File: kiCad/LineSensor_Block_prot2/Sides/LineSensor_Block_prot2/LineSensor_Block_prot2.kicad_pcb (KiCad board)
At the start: 2 copper layers, 91.3 x 94.2 mm, 58 parts, among them J1 Conn_01x09_Socket, J10 Conn_01x03_Socket, J11 Conn_01x03_Socket, J12 Conn_01x03_Socket, J2 Conn_01x09_Socket, J9 Conn_01x03_Socket, Q1 Q_Photo_NPN, Q10 Q_Photo_NPN, Q11 Q_Photo_NPN, Q12 Q_Photo_NPN, Q2 Q_Photo_NPN, Q3 Q_Photo_NPN, Q4 Q_Photo_NPN, Q5 Q_Photo_NPN, Q6 Q_Photo_NPN, Q7 Q_Photo_NPN, Q8 Q_Photo_NPN, Q9 Q_Photo_NPN

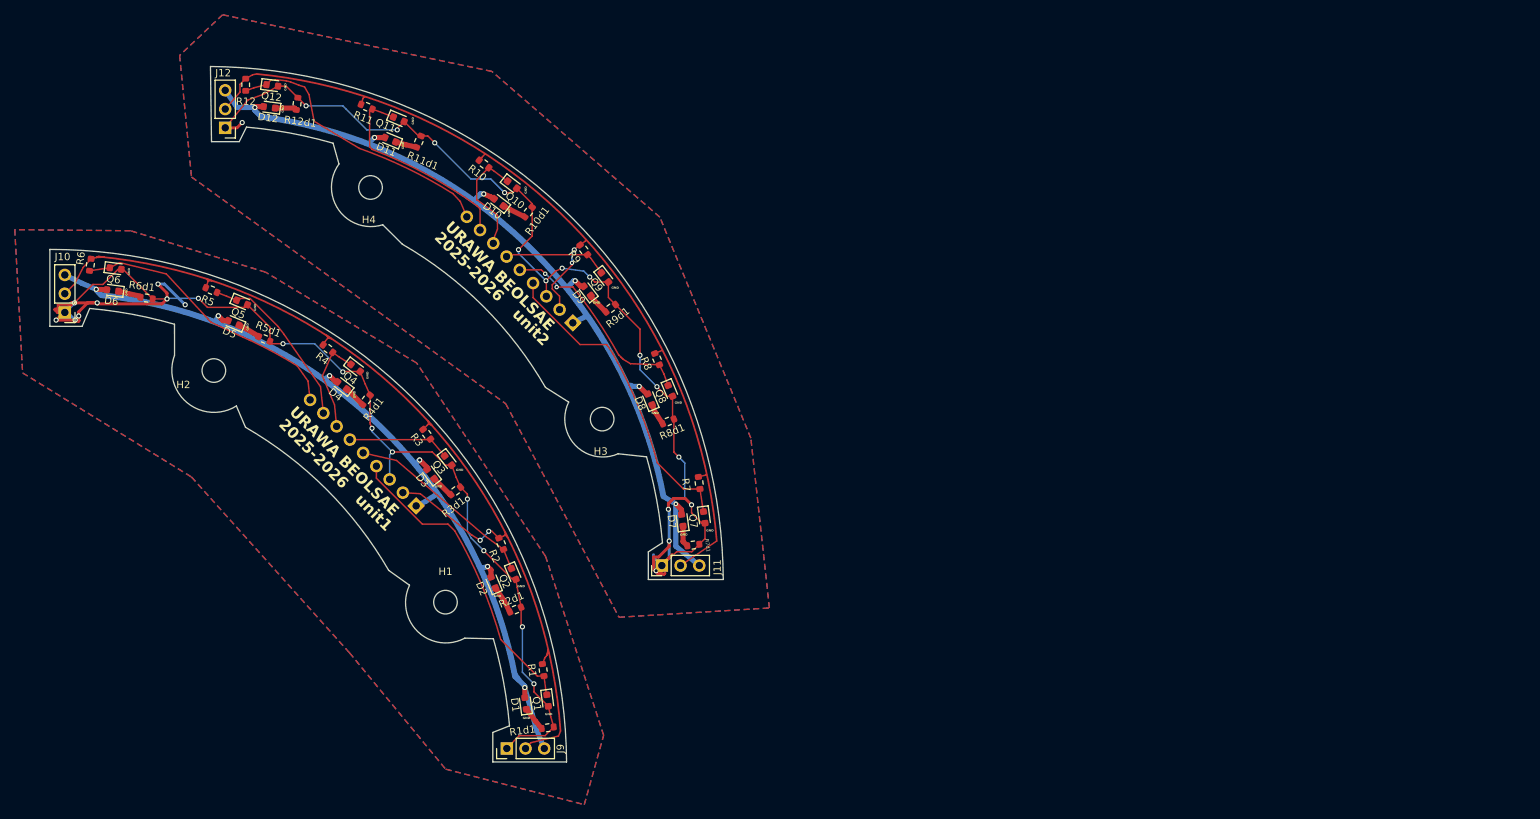
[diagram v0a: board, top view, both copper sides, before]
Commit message: ふぉるだ
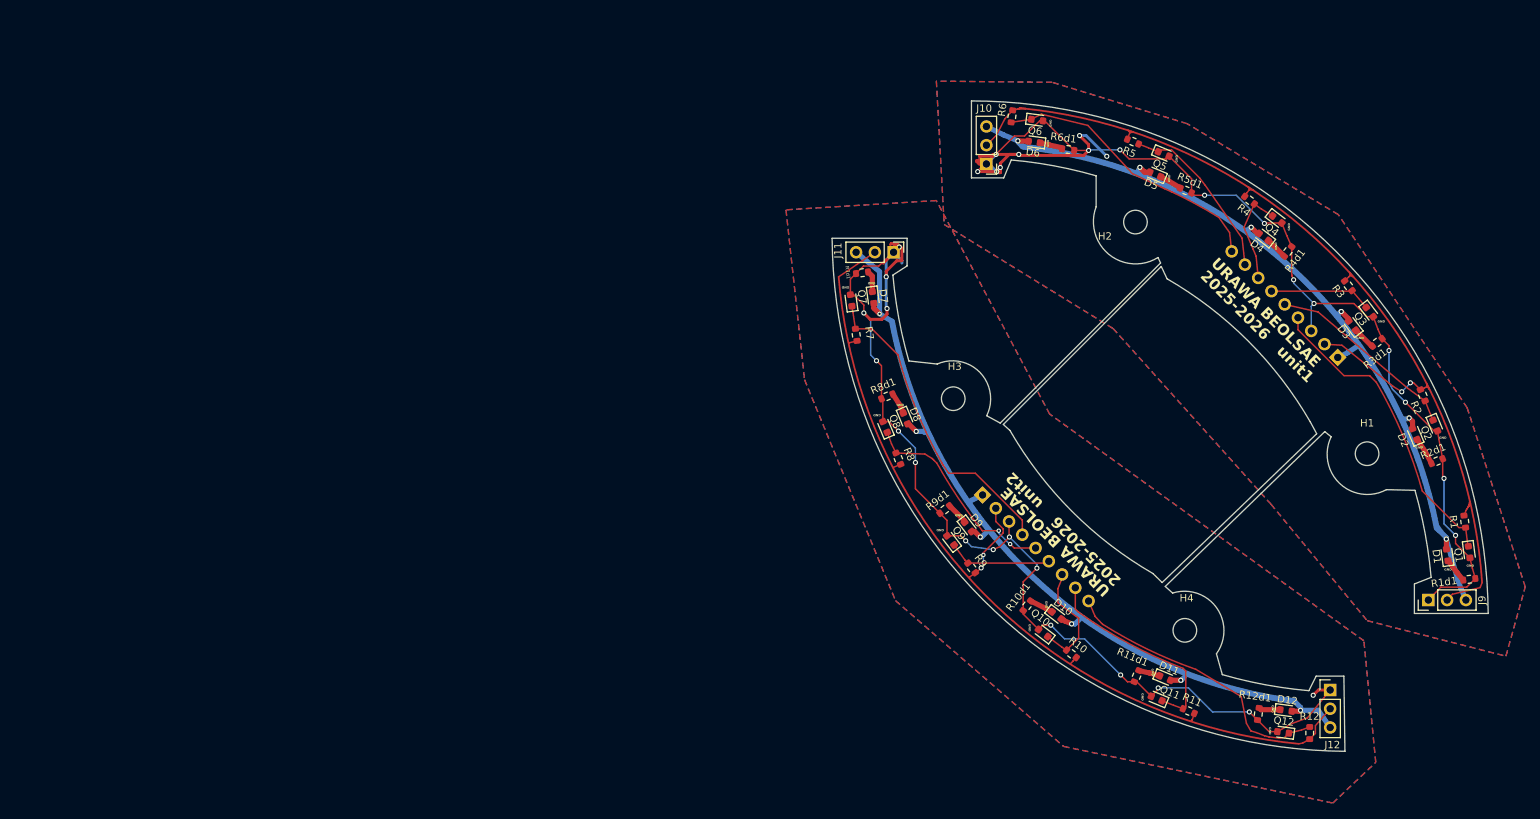
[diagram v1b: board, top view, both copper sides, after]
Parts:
- moved J12 170.4 mm to (206.4, 131.7), turned to 0 degrees
- moved R12 168.8 mm to (203.7, 135.0), turned to 90 degrees
- moved Q12 162.7 mm to (200.1, 134.9), turned to 172.5 degrees
- moved D12 160.2 mm to (200.5, 131.9), turned to -7.5 degrees
- moved R12d1 154.3 mm to (196.7, 132.4), turned to -97.5 degrees
- moved R11 138.3 mm to (187.3, 132.0), turned to 157.5 degrees
- moved Q11 129.3 mm to (182.9, 130.3), turned to 157.5 degrees
- moved D11 127.9 mm to (184.1, 127.6), turned to -22.5 degrees
- moved D1 126.5 mm to (222.3, 110.9)
- moved D5 126.5 mm to (182.7, 59.3)
- moved H1 126.5 mm to (211.4, 97.2)
- moved J1 126.5 mm to (200.3, 76.9)
- moved Q1 126.5 mm to (225.3, 110.5)
- moved Q3 126.5 mm to (211.8, 78.0)
- moved R2 126.5 mm to (219.0, 89.2)
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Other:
- board size 91.3 x 94.2 mm -> 88.9 x 88.1 mm
